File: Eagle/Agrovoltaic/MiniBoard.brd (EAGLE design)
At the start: 149.9 x 199.4 mm, 99 parts, among them J1 WAGO-03BE, J2 WAGO-03BE, J3 WAGO-03BE, K1 SRD-05VDC-SL-C, K3 SRD-05VDC-SL-C, Q1 BC338, Q2 BC338, U1 ESP32-DEVKIT-V1

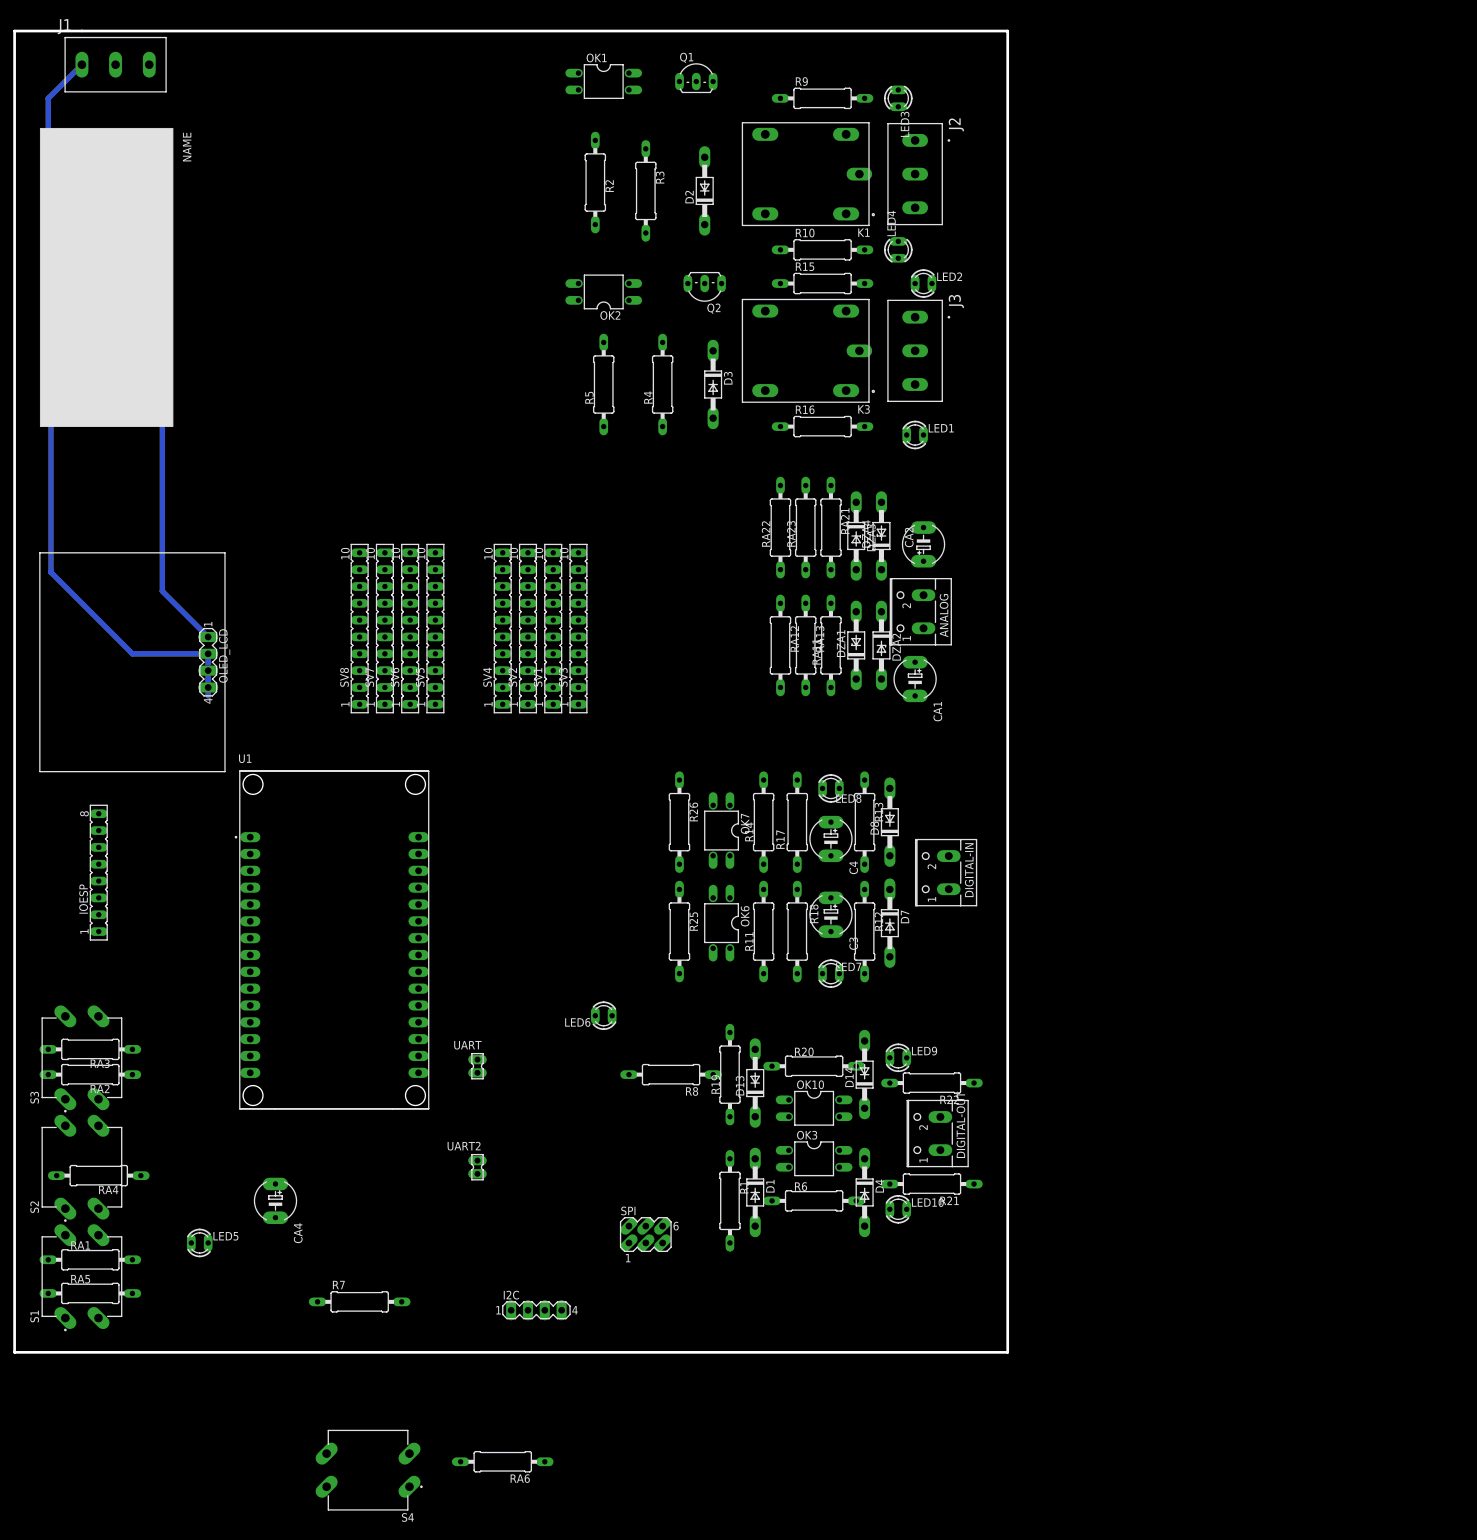
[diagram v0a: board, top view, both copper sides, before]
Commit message: MODIFY:Memisahkan Space Board
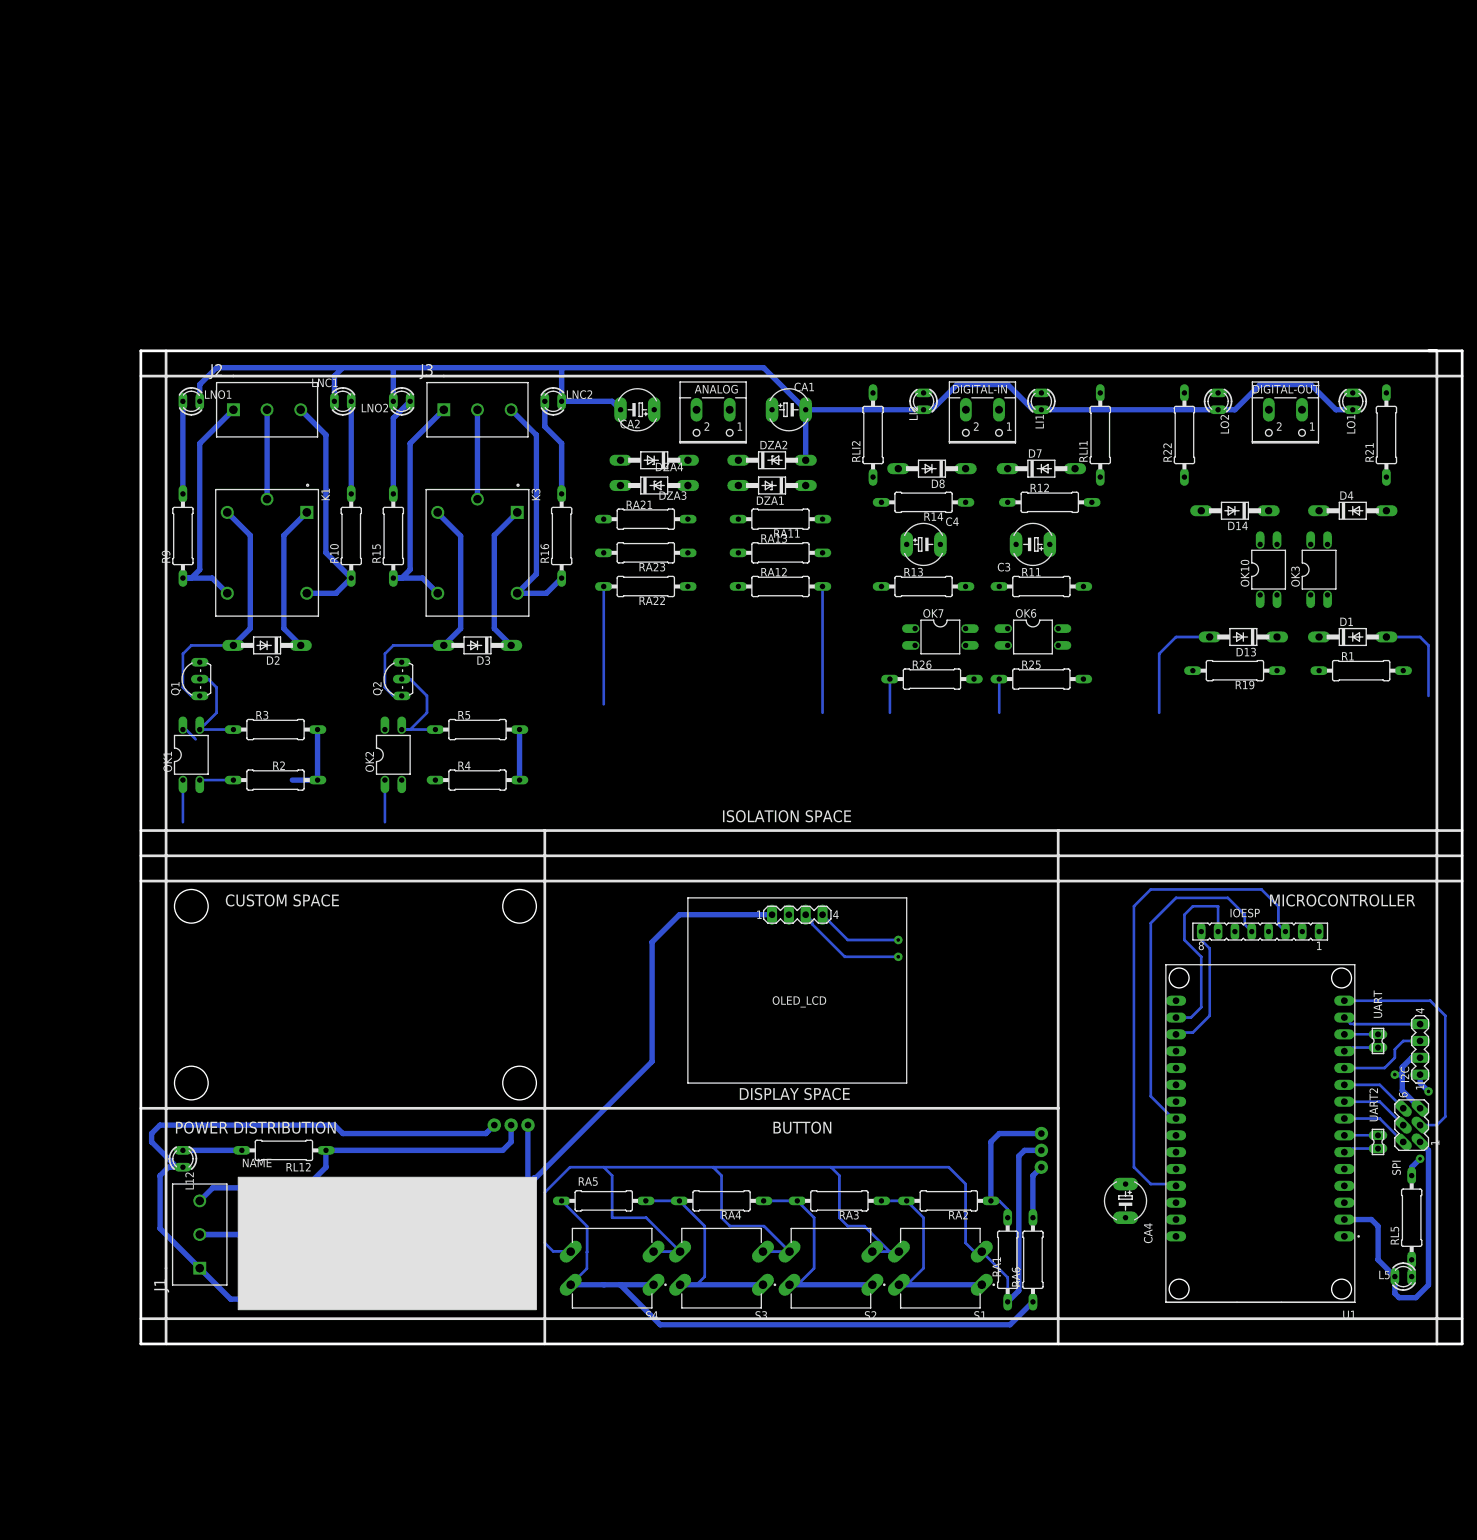
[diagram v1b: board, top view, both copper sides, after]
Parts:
- removed LED1, LED10, LED2, LED3, LED4, LED5, LED6, LED7, LED8, LED9: (no value), led_WS:LED3MM
- removed R17, R18, R7, R8: (no value), rcl-ws:0309/12
- removed R20, R6: 220, rcl-ws:0309/12
- removed SV1, SV2, SV3, SV4, SV5, SV6, SV7, SV8: (no value), con-lsta:FE10
- added L12, L5, LI1, LI2, LNC1, LNC2, LNO1, LNO2, LO1, LO2: (no value), led_WS:LED3MM
- added RL12, RL5, RLI1, RLI2: (no value), rcl-ws:0309/12
- moved J1 182.5 mm to (8.89, 11.4), turned to 90 degrees
- moved IOESP 175.5 mm to (168.9, 62.2), turned to 180 degrees
- moved U$1 149.5 mm to (38.1, 16.5), turned to 0 degrees
- moved U1 142.7 mm to (168.9, 31.8), turned to 180 degrees
- moved I2C 139.0 mm to (193.0, 44.5), turned to 90 degrees
- moved RA1 138.4 mm to (130.8, 12.7), turned to 270 degrees
- moved UART 135.9 mm to (186.7, 45.7)
- moved UART2 135.9 mm to (186.7, 30.5)
- moved R21 132.2 mm to (188.0, 137.2), turned to 90 degrees
- moved RA2 130.9 mm to (121.9, 21.6)
- moved S1 129.5 mm to (120.7, 11.4), turned to 180 degrees
- moved CA4 128.3 mm to (148.6, 21.6)
- moved D4 126.5 mm to (182.9, 125.7), turned to 0 degrees
- moved R1 124.4 mm to (184.2, 101.6), turned to 0 degrees
- moved D1 123.1 mm to (182.9, 106.7), turned to 0 degrees
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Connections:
- removed net N$17: D4.A, R6.2
- removed net N$28: D14.A, R20.2
- net 12V: now also D14.A, D2.C, D3.C, D4.A, K1.A1, K3.A1, OK1.4, OK2.4, RL12.1; no longer R20.1, R6.1, R8.1
- net 3V3: now also RA6.2
- net 5V: now also RL5.2; no longer D2.C, D3.C, K1.A1, K3.A1, OK1.4, OK2.4, R7.2
- net D4: now also RA1.2; no longer RA4.2
- net GND: now also L12.K, L5.K, LI1.K, LI2.K, LNC1.K, LNC2.K, LNO1.K, LNO2.K, LO1.K, LO2.K, RA1.1, RA2.1; no longer LED1.K, LED10.K, LED2.K, LED3.K, LED4.K, LED5.K, LED6.K, LED7.K, LED8.K, LED9.K, RA3.1, RA4.1
- net N$10: now also LNO2.A; no longer LED2.A
- net N$11: now also LNC2.A; no longer LED1.A
- net N$12: now also LNO1.A; no longer LED3.A
- net N$13: now also LNC1.A; no longer LED4.A
- net N$14: now also L12.A, RL12.2; no longer LED6.A, R8.2
- net N$19: now also RLI1.1; no longer R18.1
- net N$21: now also RLI2.1; no longer R17.1
- net N$23: now also L5.A, RL5.1; no longer LED5.A, R7.1
- net N$24: now also LI2.A, RLI2.2; no longer LED8.A, R17.2
- net N$29: now also LI1.A, RLI1.2; no longer LED7.A, R18.2
- net N$30: now also LO1.A; no longer LED10.A
- net N$31: now also LO2.A; no longer LED9.A
- net N$5: now also RA4.2, S3.1, S3.2; no longer RA1.2, S1.1, S1.2
- net N$8: now also RA3.2, RA4.1; no longer RA1.1, RA2.2
- net N$9: now also RA2.2, RA3.1, S1.1, S1.2; no longer RA2.1, RA3.2, S3.1, S3.2
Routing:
- net GND: track 114.0 -> 441.2 mm, vias 0 -> 3
- net D4: track 0.11 -> 196.8 mm, vias 0 -> 1
- net 5V: track 36.2 -> 174.4 mm, vias 0 -> 3
- net 12V: track 0.00 -> 102.4 mm, vias 0 -> 1
- net N$32: track 0.00 -> 94.0 mm
- net D12: track 0.00 -> 75.2 mm
- net D25: track 0.00 -> 51.1 mm
- net N$7: track 0.00 -> 40.1 mm
- net N$4: track 0.00 -> 38.8 mm
- net NC2: track 0.00 -> 38.1 mm
- net NO2: track 0.00 -> 36.9 mm
- net NO1: track 0.00 -> 36.9 mm
- net NC1: track 0.00 -> 36.2 mm
- net MOSI: track 0.00 -> 35.8 mm
- net N$5: track 0.00 -> 34.8 mm
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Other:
- board size 149.9 x 199.4 mm -> 199.4 x 149.9 mm
- board text added: "BUTTON"
- board text added: "CUSTOM SPACE"
- board text added: "DISPLAY SPACE"
- board text added: "ISOLATION SPACE"
- board text added: "MICROCONTROLLER"
- board text added: "POWER DISTRIBUTION"
